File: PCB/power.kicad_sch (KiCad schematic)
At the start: 23 parts, among them U2 LTC3370

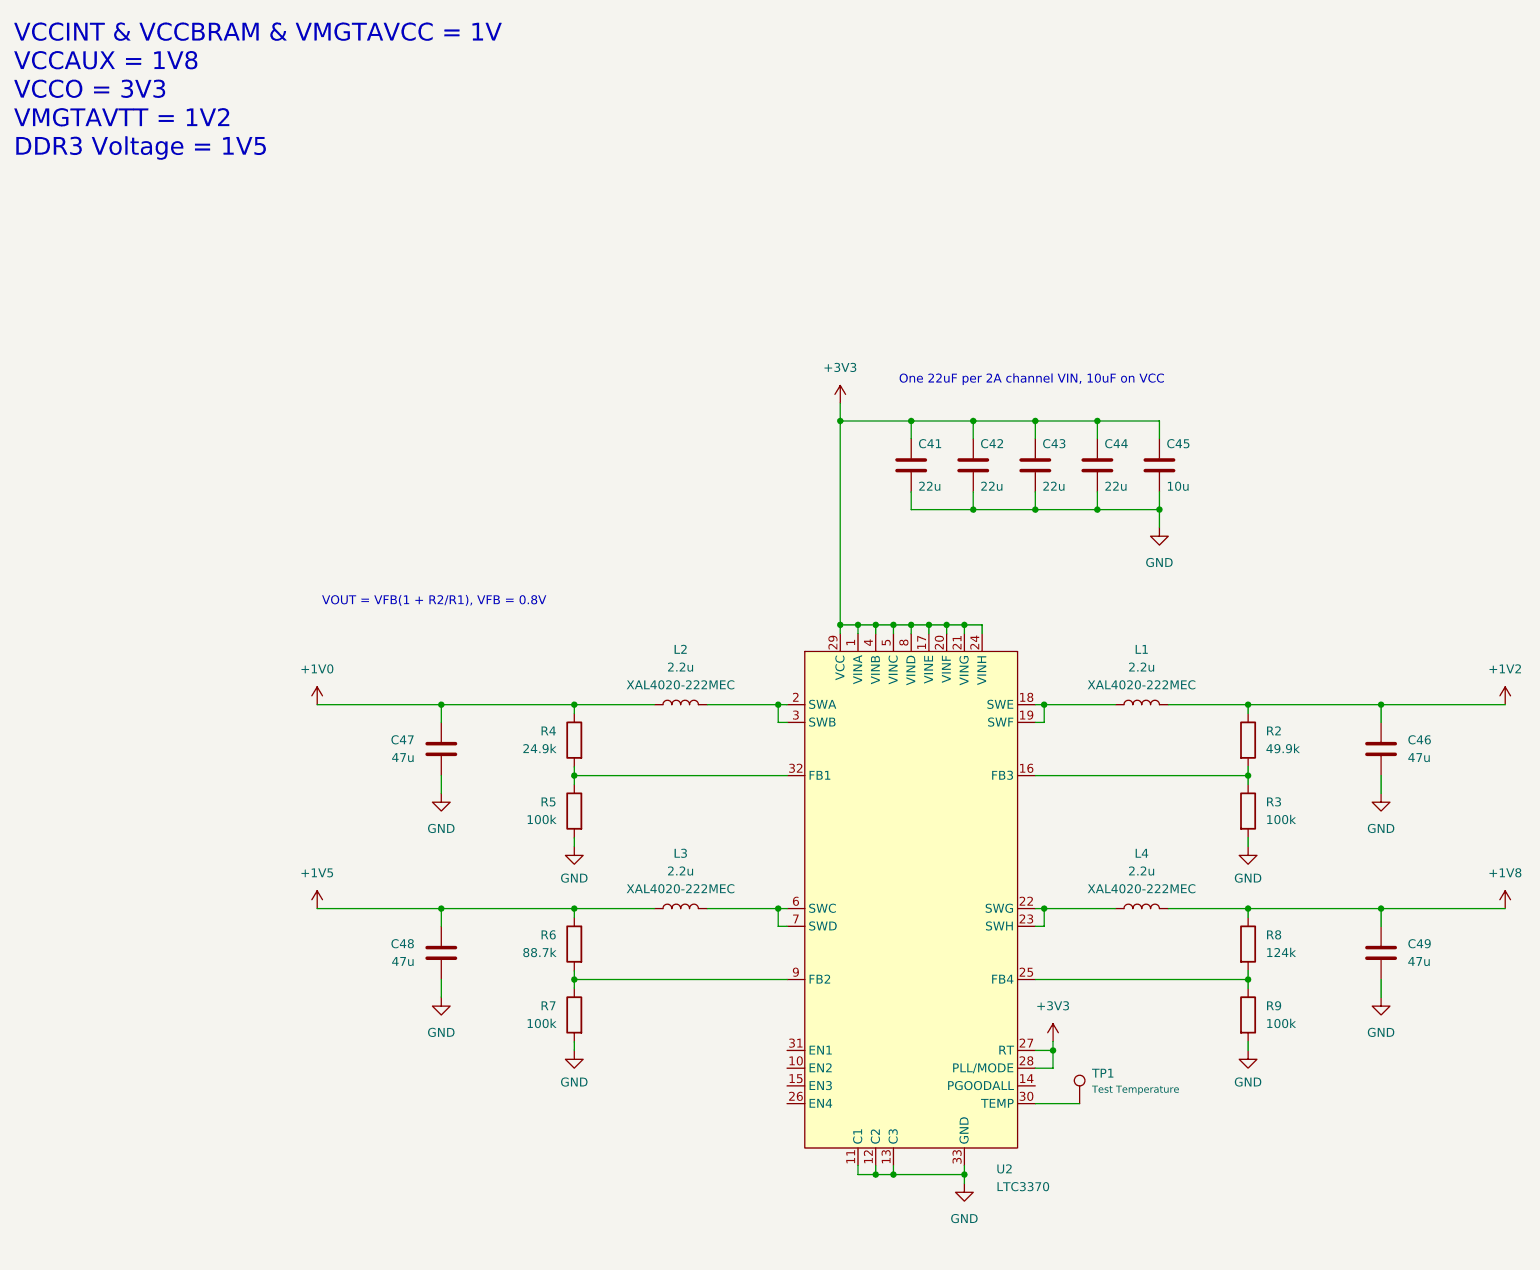
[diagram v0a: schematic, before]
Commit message: custom MAX20029 symbol
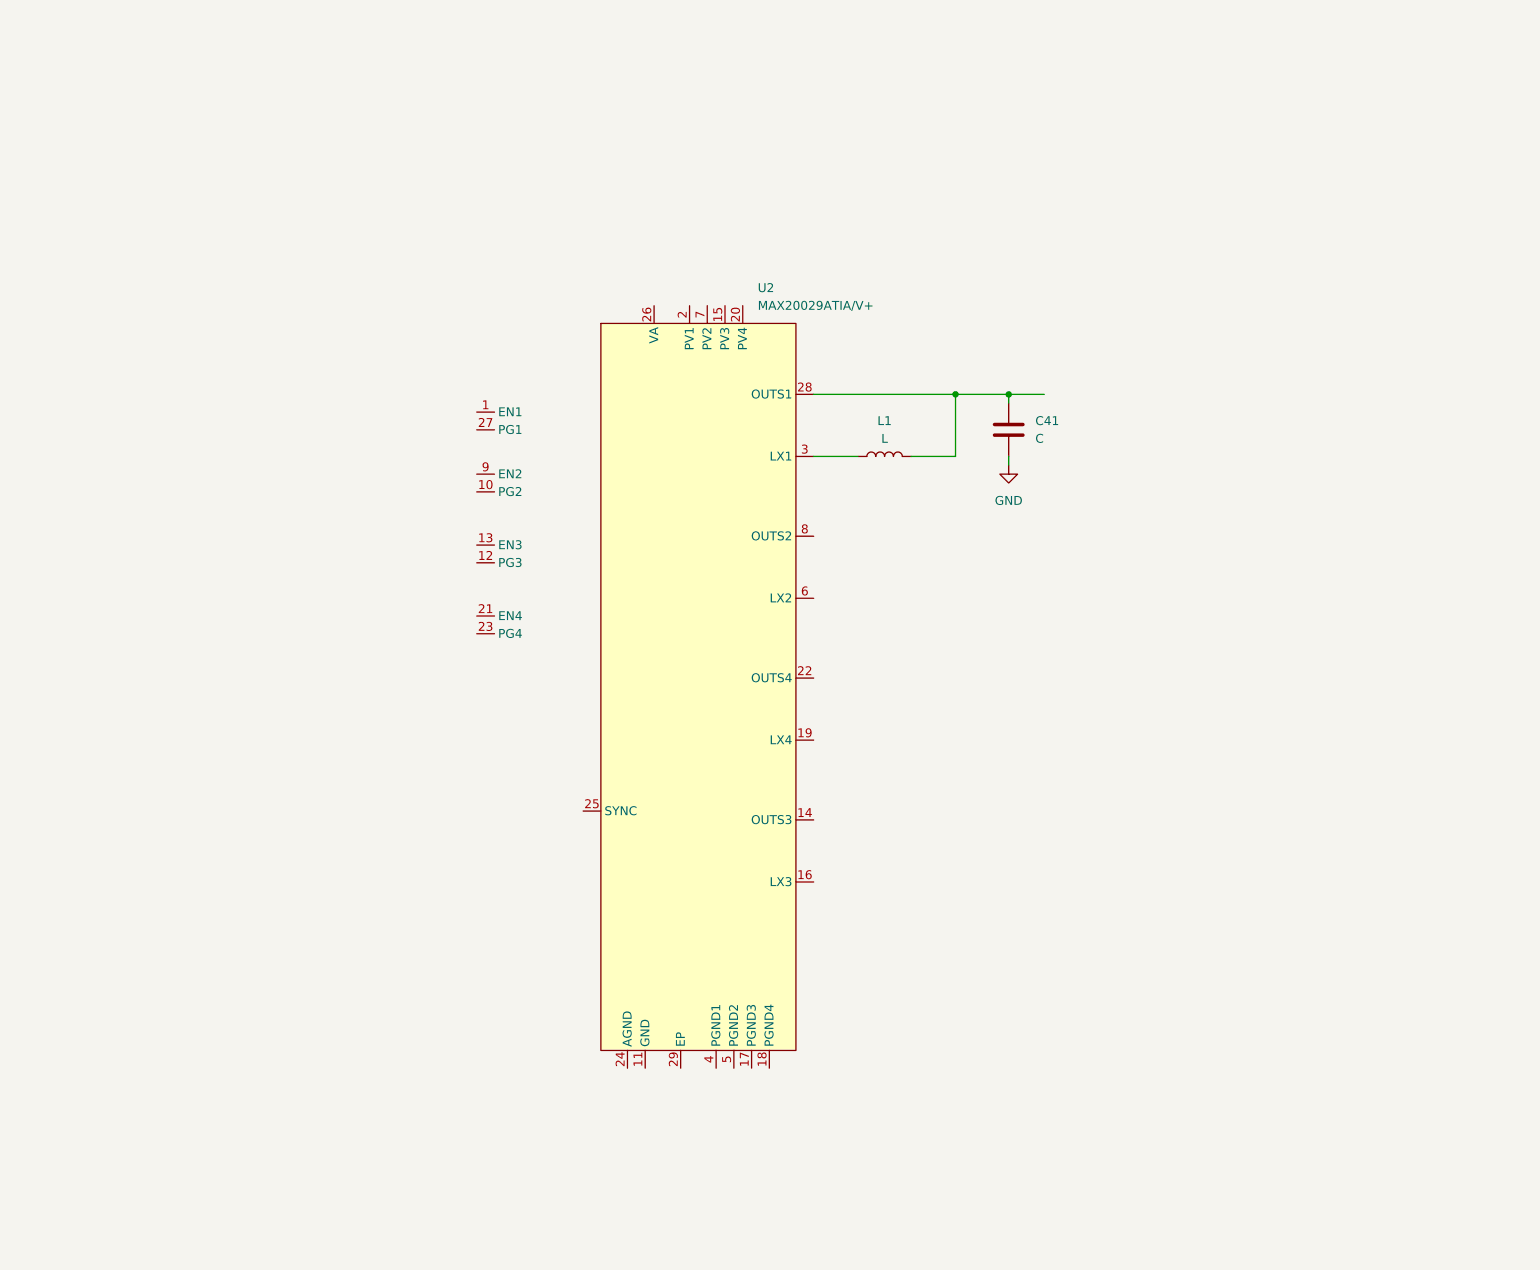
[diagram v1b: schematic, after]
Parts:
- removed C42, C43, C44: 22u, symbol Device:C
- removed C45: 10u, symbol Device:C
- removed C46, C47, C48, C49: 47u, symbol Device:C
- removed L2, L3, L4: 2.2u, symbol Device:L
- removed R2: 49.9k, symbol Device:R
- removed R3, R5, R7, R9: 100k, symbol Device:R
- removed R4: 24.9k, symbol Device:R
- removed R6: 88.7k, symbol Device:R
- removed R8: 124k, symbol Device:R
- removed TP1: Test Temperature, symbol Connector:TestPoint
- removed U2: LTC3370, Package_DFN_QFN:QFN-32-1EP_5x5mm_P0.5mm_EP3.45x3.45mm_ThermalVias, symbol FPGA Accelerator:LTC3370
- added U2: MAX20029ATIA/V+, easyeda2kicad:QFN-28_L5.0-W5.0-P0.50-TL-EP3.2, symbol FPGA Accelerator:MAX20029
- C41: value 22u -> C
- L1: value 2.2u -> L; DK P# 2457-XAL4020-222MEC-ND -> (none); LCSC C3151182 -> (none); MPN XAL4020-222MEC -> (none)
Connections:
- net +3V3 is gone; now on an unnamed net: C41.1
- net at L1.1: now also U2.3 (LX1)
- net +1V2: no longer names the net of L1.2
- net +1V2: now also U2.28 (OUTS1)
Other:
- note removed: "One 22uF per 2A channel VIN, 10uF on VCC"
- note removed: "VCCINT & VCCBRAM & VMGTAVCC = 1V VCCAUX = 1V8 VCCO = 3V3 VMGTAVTT = 1V2 DDR3 Voltage = 1V5"
- note removed: "VOUT = VFB(1 + R2/R1), VFB = 0.8V"

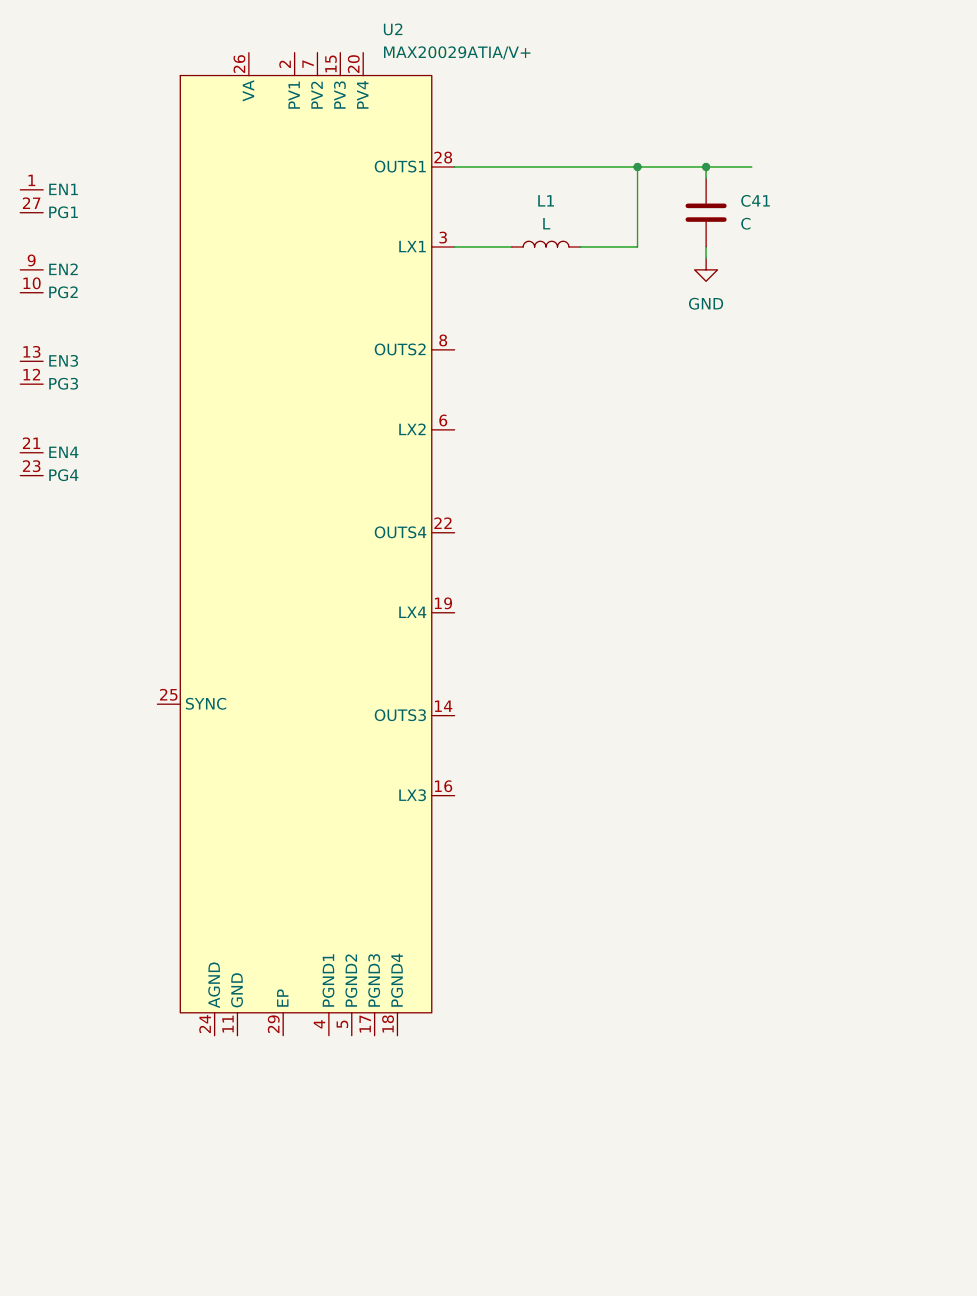
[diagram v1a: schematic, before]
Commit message: halfway done buck wiring
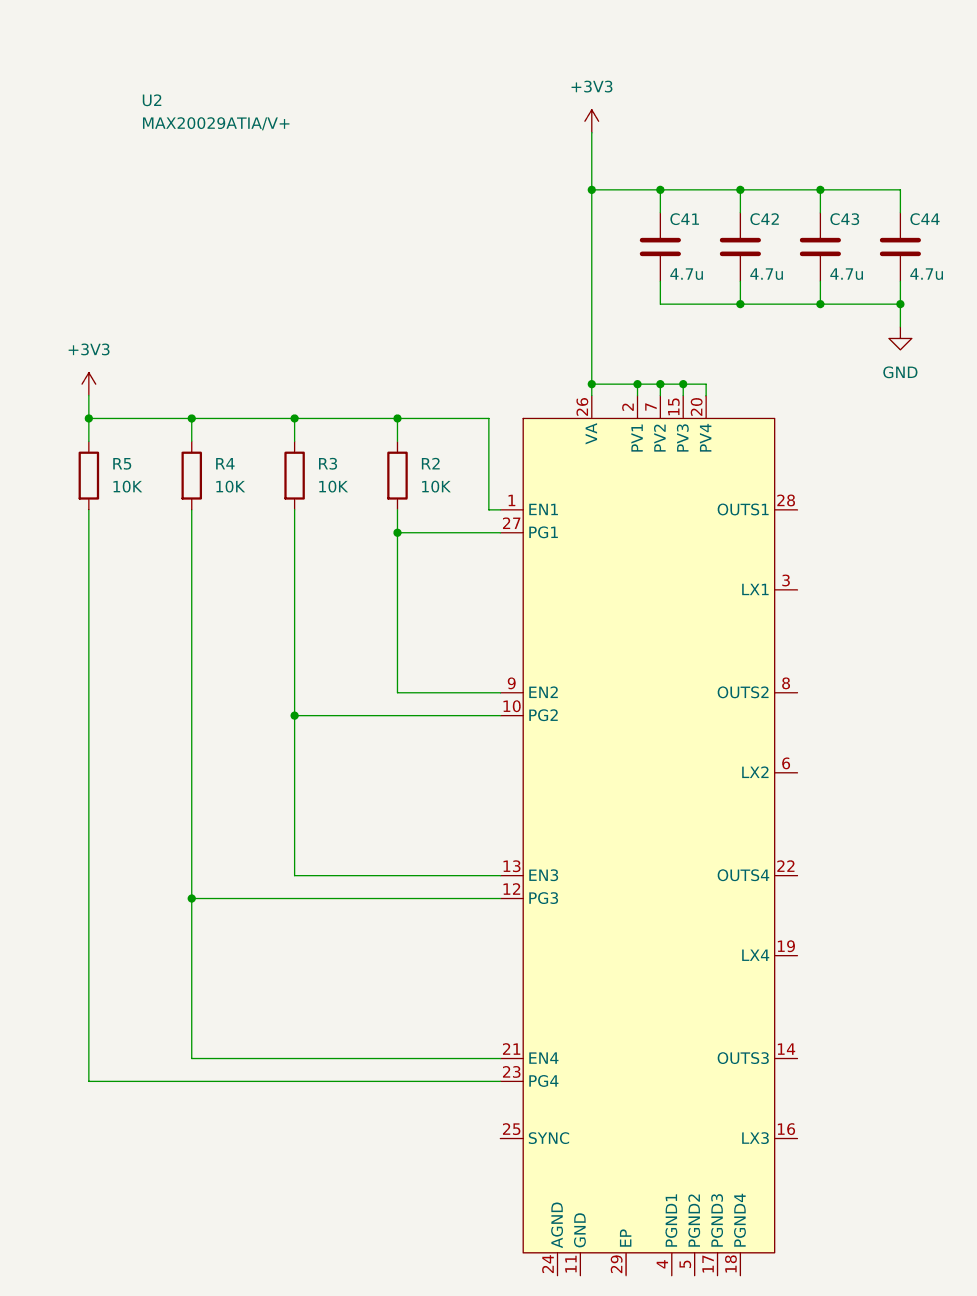
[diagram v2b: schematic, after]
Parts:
- removed L1: L, symbol Device:L
- added C42, C43, C44: 4.7u, symbol Device:C
- added R2, R3, R4, R5: 10K, symbol Device:R
- C41: value C -> 4.7u
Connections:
- net GND: now also C42.2, C43.2, C44.2
- net at U2.28 (OUTS1): no longer C41.1
- net +3V3: now reaches U2.1 (EN1)
- net +3V3: now also C41.1, U2.15 (PV3), U2.2 (PV1), U2.20 (PV4), U2.26 (VA), U2.7 (PV2), C42.1, C43.1, C44.1, R2.1, R3.1, R4.1, R5.1
- net at U2.10 (PG2): now also U2.13 (EN3), R3.2
- net at U2.12 (PG3): now also U2.21 (EN4), R4.2
- net at U2.23 (PG4): now also R5.2
- net at U2.27 (PG1): now also U2.9 (EN2), R2.2
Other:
- moved on the sheet: U2
